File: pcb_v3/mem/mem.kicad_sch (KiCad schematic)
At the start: 27 parts, among them J1 bus mem, J2 bus mem, J3 cartridge, U1 CY62256-70PC, U2 CY62256-70PC, U3 74LS283, U4 74LS00, U5 74LS32, U7 74LS138

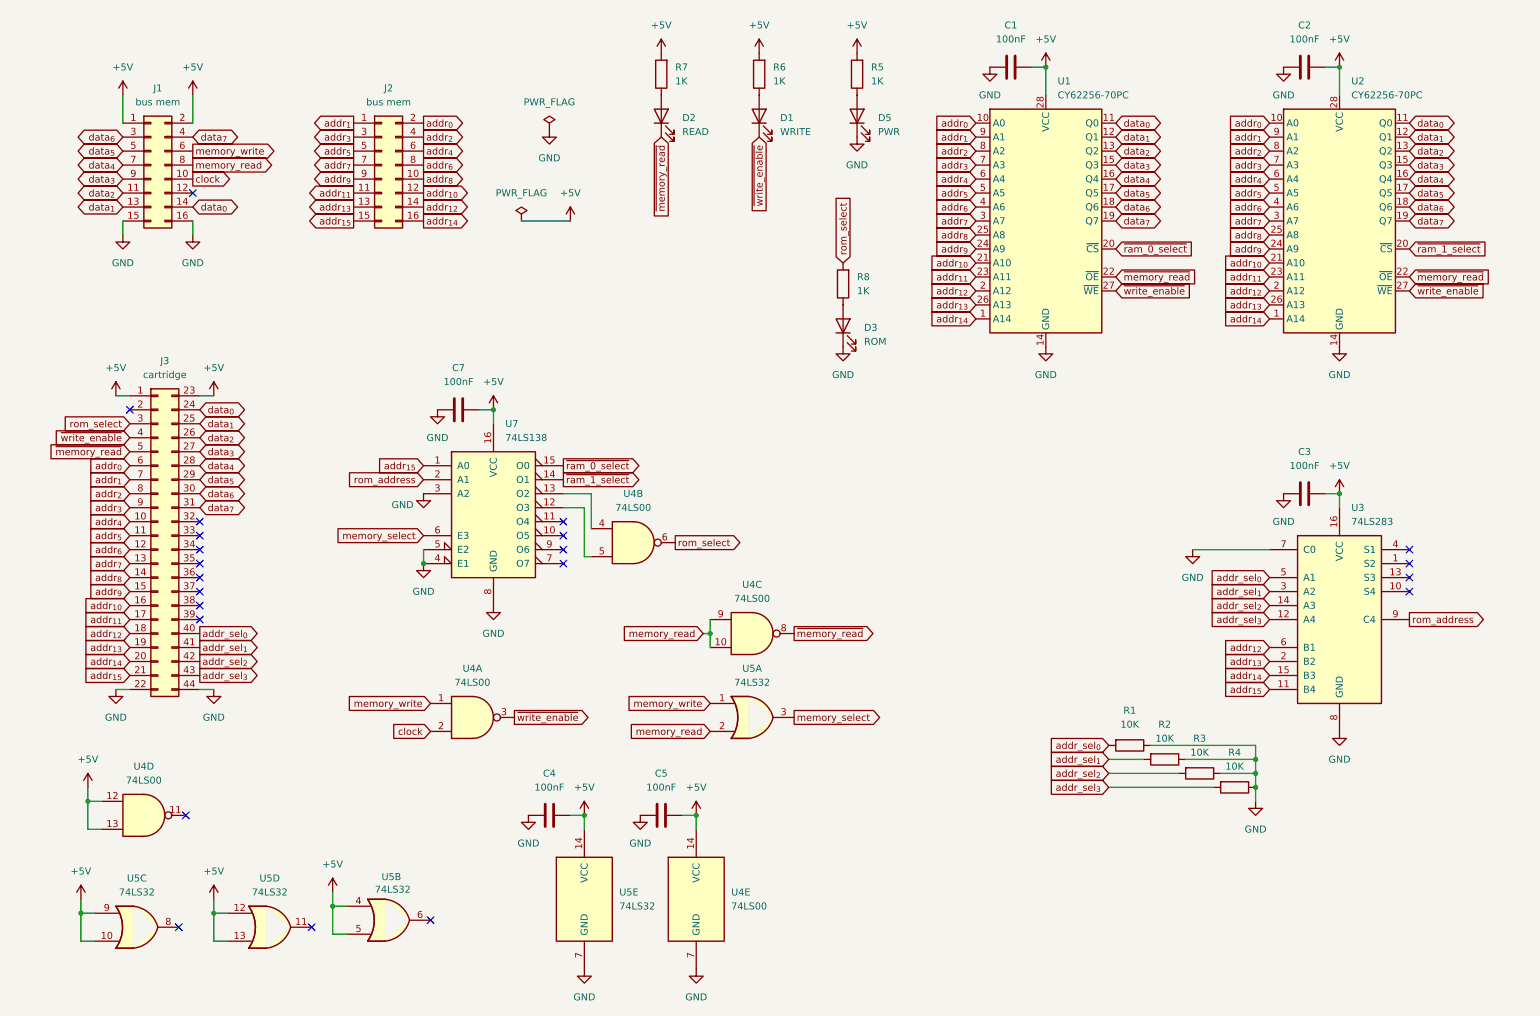
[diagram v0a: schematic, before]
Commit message: avançando no layot v3
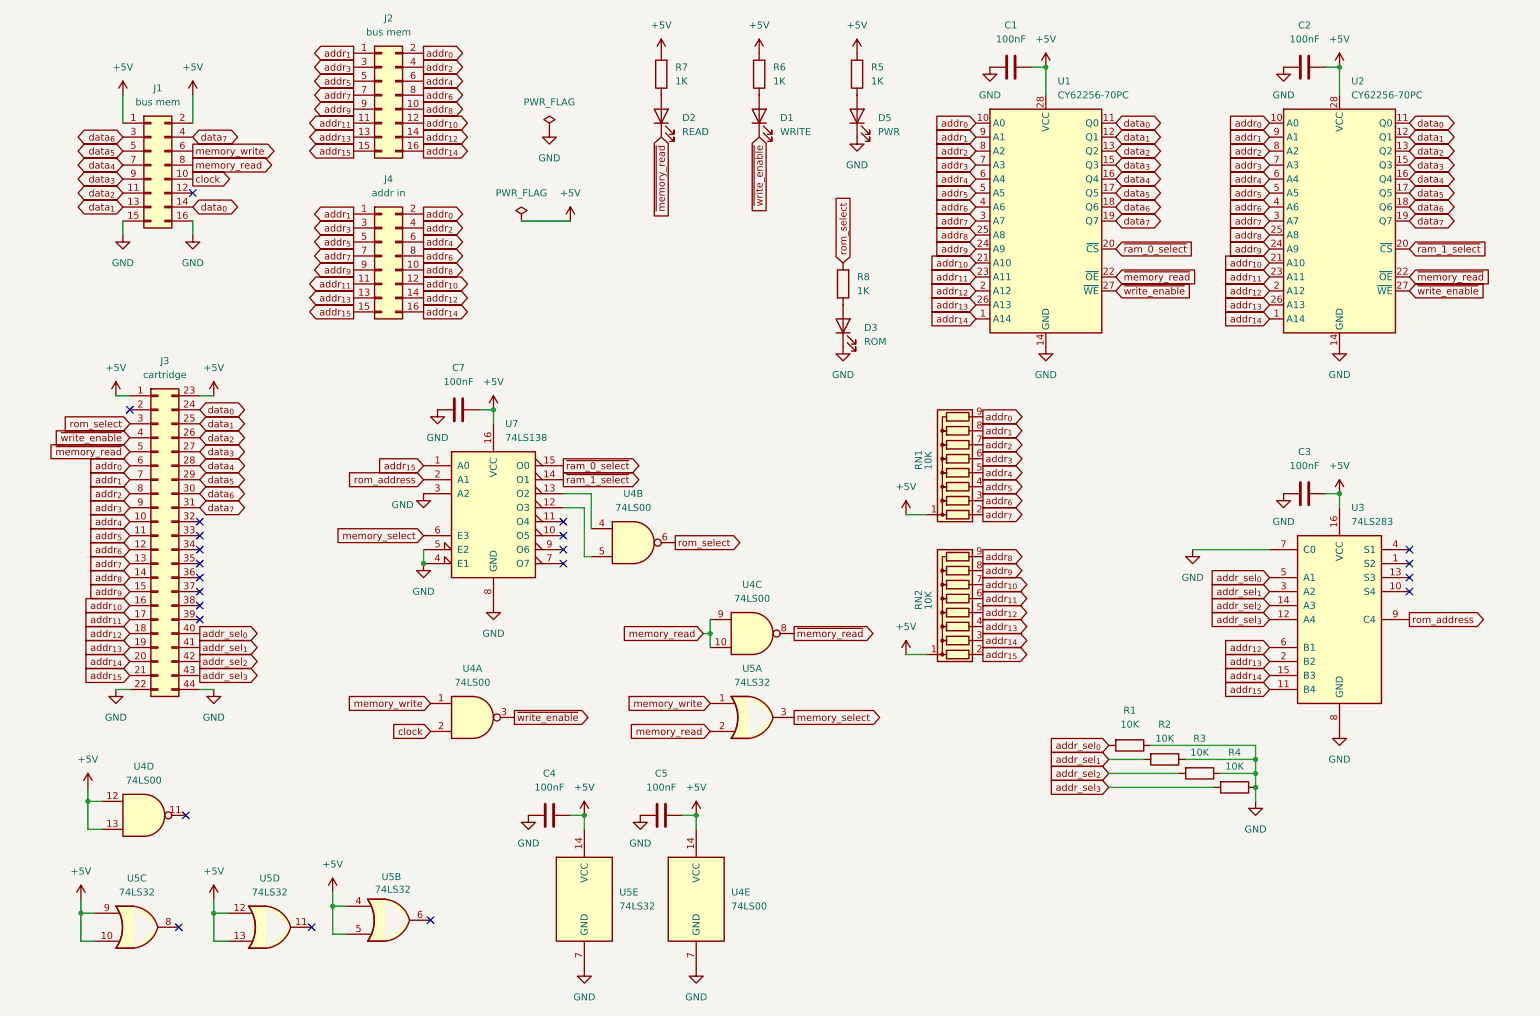
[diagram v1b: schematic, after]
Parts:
- added J4: addr in, edge_connector:conector 02x08, symbol Connector_Generic:Conn_02x08_Odd_Even
- added RN1, RN2: 10K, Resistor_THT:R_Array_SIP9, symbol Device:R_Network08
- J1, J2: footprint Connector_PinHeader_2.54mm:PinHeader_2x08_P2.54mm_Vertical -> edge_connector:conector 02x08
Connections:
- net +5V: now also RN1.1 (common), RN2.1 (common)
- net addr_{0}: now also J4.2 (Pin_2), RN1.9 (R8)
- net addr_{10}: now also J4.12 (Pin_12), RN2.7 (R6)
- net addr_{11}: now also J4.11 (Pin_11), RN2.6 (R5)
- net addr_{12}: now also J4.14 (Pin_14), RN2.5 (R4)
- net addr_{13}: now also J4.13 (Pin_13), RN2.4 (R3)
- net addr_{14}: now also J4.16 (Pin_16), RN2.3 (R2)
- net addr_{15}: now also J4.15 (Pin_15), RN2.2 (R1)
- net addr_{1}: now also J4.1 (Pin_1), RN1.8 (R7)
- net addr_{2}: now also J4.4 (Pin_4), RN1.7 (R6)
- net addr_{3}: now also J4.3 (Pin_3), RN1.6 (R5)
- net addr_{4}: now also J4.6 (Pin_6), RN1.5 (R4)
- net addr_{5}: now also J4.5 (Pin_5), RN1.4 (R3)
- net addr_{6}: now also J4.8 (Pin_8), RN1.3 (R2)
- net addr_{7}: now also J4.7 (Pin_7), RN1.2 (R1)
- net addr_{8}: now also J4.10 (Pin_10), RN2.9 (R8)
- net addr_{9}: now also J4.9 (Pin_9), RN2.8 (R7)
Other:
- moved on the sheet: J2
